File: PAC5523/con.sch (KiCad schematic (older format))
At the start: 43 parts, among them J10 NTC, J11 LED, J4 GND, J5 VIN, J6 UART, J8 HALL, J9 LED, P1 TC2030-CTX-Tag-Connect, Q2 Q_NMOS_GSD

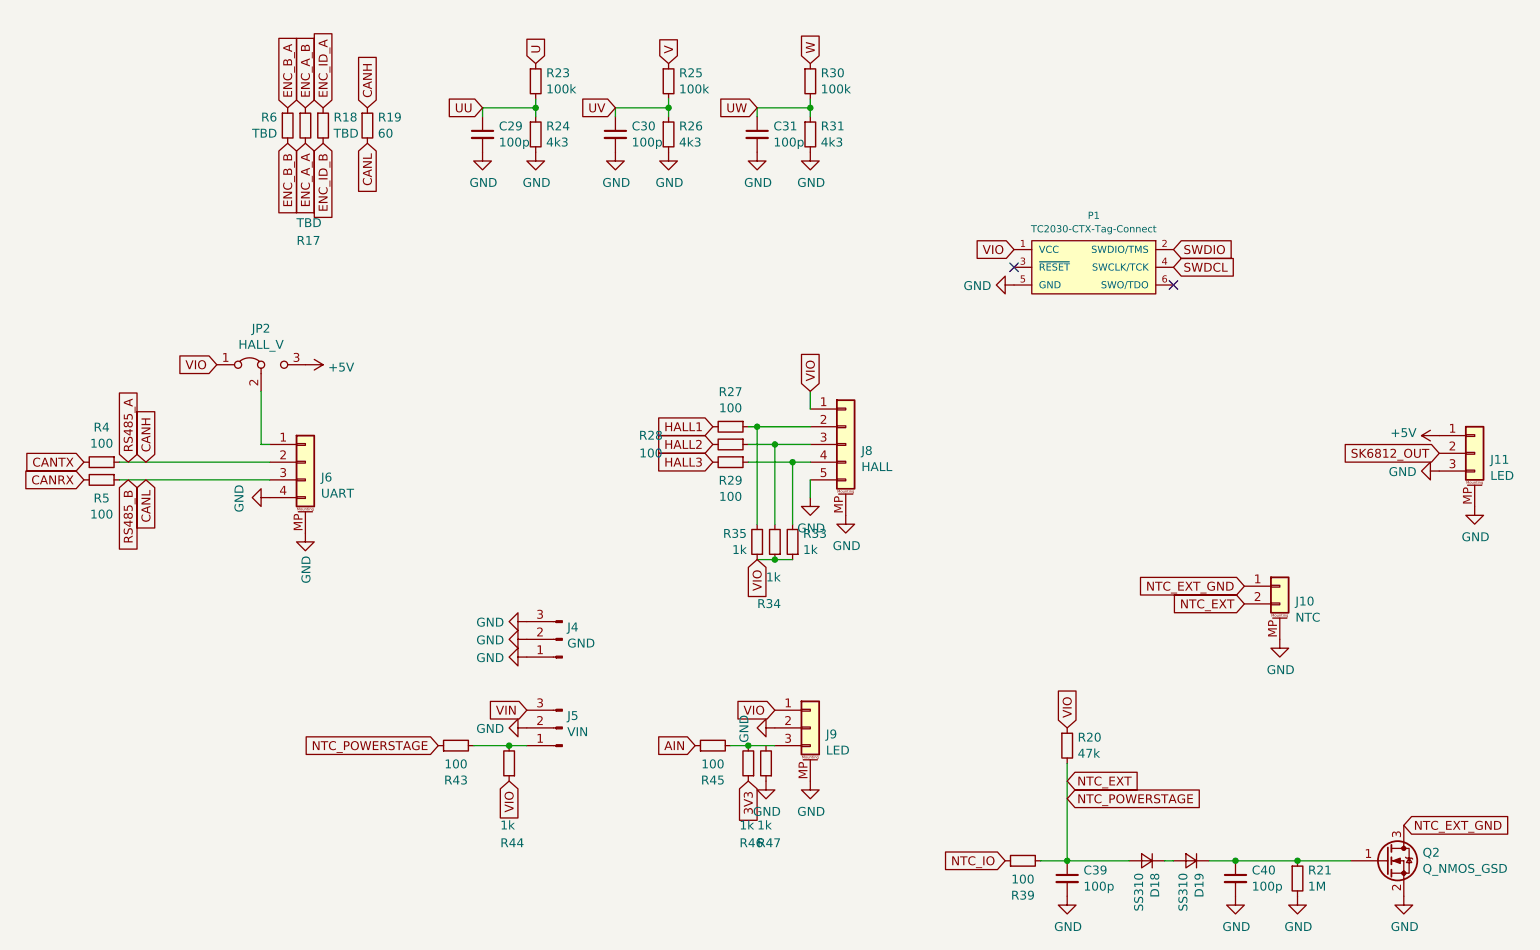
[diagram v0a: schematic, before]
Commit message: placement almost done
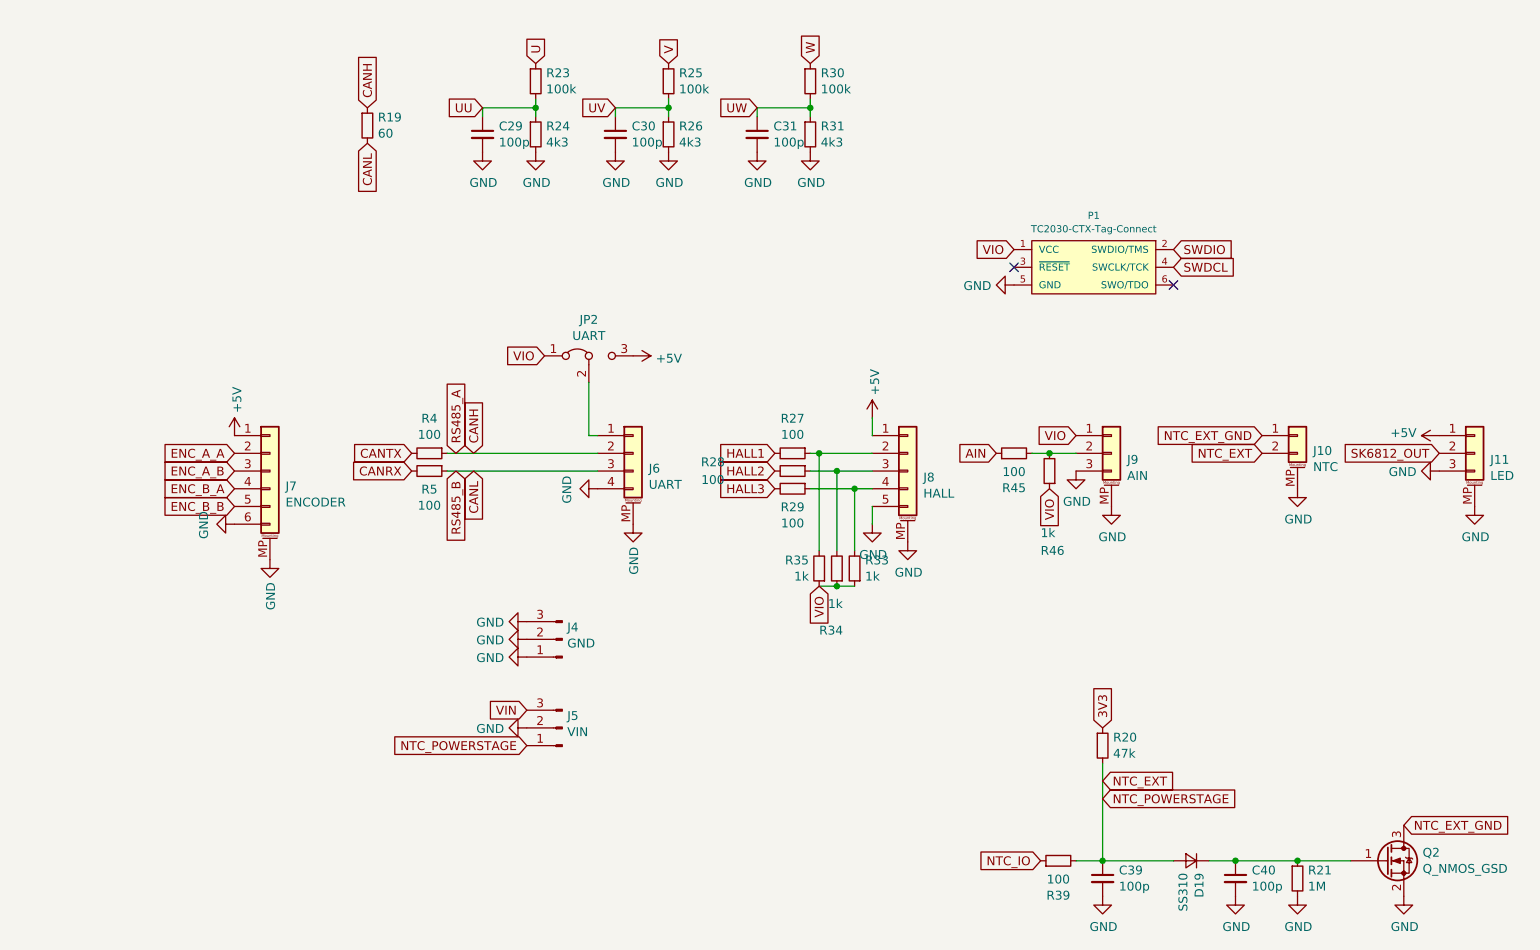
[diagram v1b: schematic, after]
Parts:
- removed D18: SS310, Diode_SMD:D_SOD-123F, symbol Device:D_Small
- removed R17, R18, R6: TBD, Resistor_SMD:R_0603_1608Metric, symbol Device:R_Small
- removed R43: 100, Resistor_SMD:R_0603_1608Metric, symbol Device:R_Small
- removed R44, R47: 1k, Resistor_SMD:R_0603_1608Metric, symbol Device:R_Small
- added J7: ENCODER, Connector_Molex:Molex_PicoBlade_53261-0671_1x06-1MP_P1.25mm_Horizontal, symbol Connector_Generic_MountingPin:Conn_01x06_MountingPin
- J9: value LED -> AIN
- JP2: value HALL_V -> UART
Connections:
- net +5V: now also J8.1 (Pin_1), J7.1 (Pin_1)
- net 3V3: now also R20.1; no longer R46.1
- net ENC_A_A: now also J7.2 (Pin_2)
- net ENC_A_B: now also J7.3 (Pin_3)
- net ENC_B_A: now also J7.4 (Pin_4)
- net ENC_B_B: now also J7.5 (Pin_5)
- net GND: now also J9.3 (Pin_3), J7.6 (Pin_6), J7.MP (MountPin); no longer J9.2 (Pin_2)
- net NTC_EXT: now also D19.2 (A), J5.1 (Pin_1)
- net VIO: now also R46.1; no longer J8.1 (Pin_1), R20.1
- net at R45.2, R46.2: now also J9.2 (Pin_2); no longer J9.3 (Pin_3)
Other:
- moved on the sheet: C39, J10, J6, J8, J9, JP2, R20, R27, R28, R29, R33, R34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
